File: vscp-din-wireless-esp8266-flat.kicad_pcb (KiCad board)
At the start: 2 copper layers, 64.8 x 51 mm, 25 parts, among them J1 Conn_01x04_Left, J2 Conn_01x04_Right, J3 Conn_01x06, J4 Conn_01x02, Q1 BC547, U2 ESP-12E

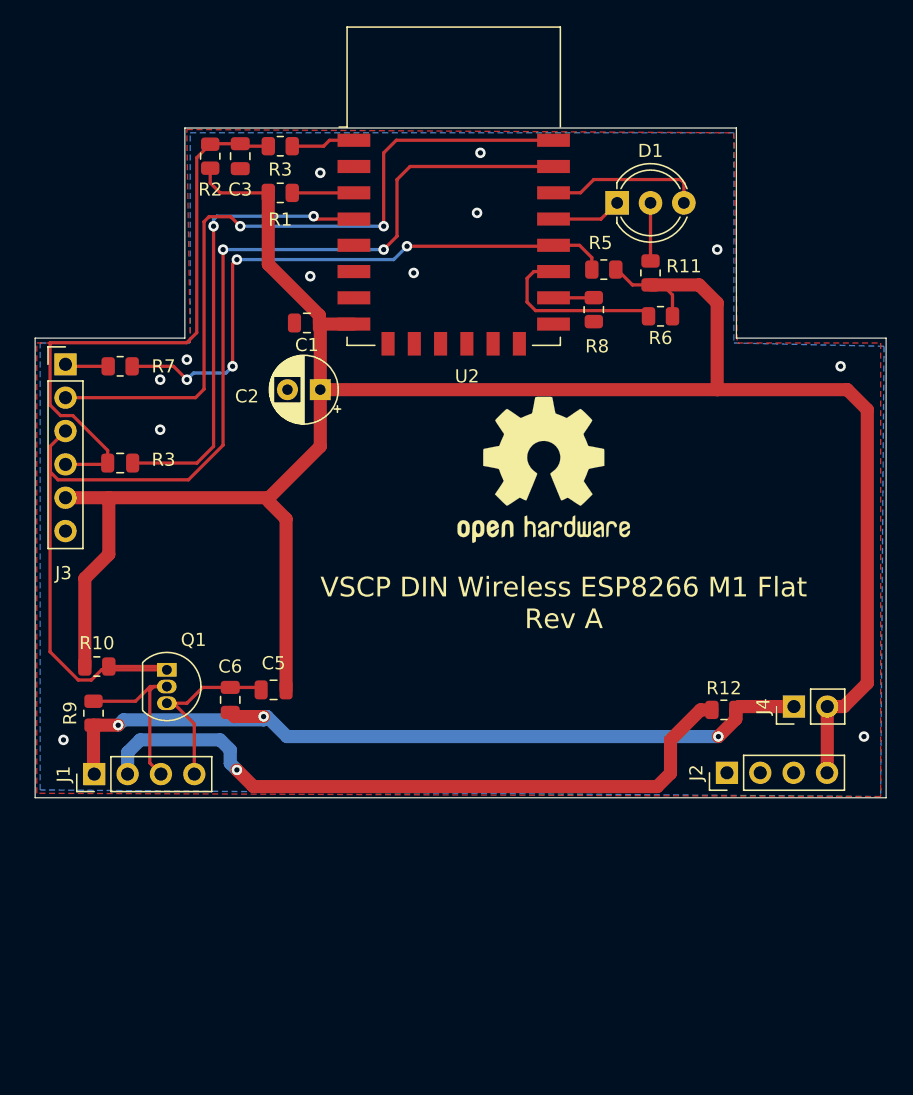
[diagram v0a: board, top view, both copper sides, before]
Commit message: Added gerbers
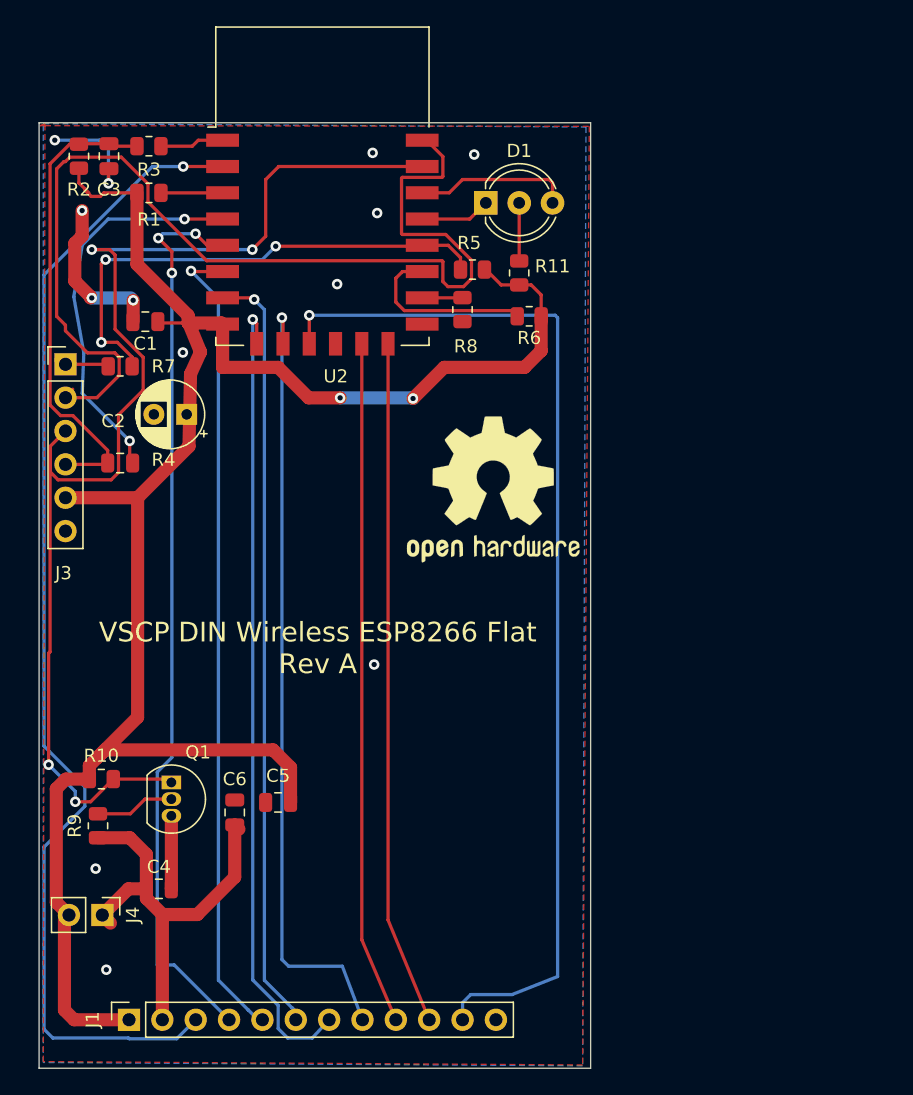
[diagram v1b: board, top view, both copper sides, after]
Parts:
- removed J2: Conn_01x04_Right, Connector_PinHeader_2.54mm:PinHeader_1x04_P2.54mm_Vertical
- removed R12: 0R, Resistor_SMD:R_0805_2012Metric
- added C4: 100nF, Capacitor_SMD:C_0805_2012Metric, F.Cu at (125.1, 106.3)
- J1: value Conn_01x04_Left -> Conn_01x12; footprint Connector_PinHeader_2.54mm:PinHeader_1x04_P2.54mm_Vertical -> Connector_PinSocket_2.54mm:PinSocket_1x12_P2.54mm_Vertical
- moved J4 55.0 mm to (120.8, 108.3), turned to 270 degrees
- moved J1 18.9 mm to (122.8, 116.3)
- moved C1 12.3 mm to (124.1, 63.1)
- moved C2 10.3 mm to (127.2, 70.2)
- moved C3 10.0 mm to (121.3, 50.5)
- moved R1 10.0 mm to (124.4, 53.3)
- moved R2 10.0 mm to (119.0, 50.5)
- moved R3 10.0 mm to (124.4, 49.8)
- moved D1 10.0 mm to (150.0, 54.1)
- moved R11 10.0 mm to (152.6, 59.4)
- moved R5 10.0 mm to (149.0, 59.2)
- moved R6 10.0 mm to (153.3, 62.7)
- moved R8 10.0 mm to (148.2, 62.2)
- moved U2 10.0 mm to (137.6, 52.8)
- moved R10 8.58 mm to (120.7, 98.0)
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- renumbered R3 to R4
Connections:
- J1 pad 1: VDD -> VCC
- J1 pad 2: Net-(J1-Pad2) -> VDD
- J1 pad 3: Net-(J1-Pad3) -> /adc
- J1 pad 4: GND -> /gpio14
- Q1 pad 2: Net-(J1-Pad3) -> /TTLRX
- R9 pad 1: Net-(J1-Pad3) -> /TTLRX
- U2 pad 10: Net-(U2-Pad10) -> /MISO
- U2 pad 11: Net-(U2-Pad11) -> /gpio9
- U2 pad 13: Net-(U2-Pad13) -> /MOSI
- U2 pad 14: Net-(U2-Pad14) -> /SCLK
- U2 pad 2: Net-(U2-Pad2) -> /adc
- U2 pad 5: Net-(U2-Pad5) -> /gpio14
- U2 pad 6: Net-(U2-Pad6) -> /gpio12
- U2 pad 7: Net-(U2-Pad7) -> /gpio13
- U2 pad 9: Net-(U2-Pad9) -> /CS0
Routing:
- net /adc: track 0.00 -> 89.5 mm, vias 0 -> 1
- net /gpio9: track 0.00 -> 80.4 mm, vias 0 -> 1
- net /gpio14: track 0.00 -> 68.8 mm, vias 0 -> 3
- net /gpio12: track 0.00 -> 61.9 mm, vias 0 -> 1
- net /CS0: track 0.00 -> 61.6 mm, vias 0 -> 1
- net /MISO: track 0.00 -> 60.1 mm, vias 0 -> 1
- net /gpio13: track 0.00 -> 58.9 mm, vias 0 -> 1
- net Net-(J1-Pad2): track 52.5 -> 0.00 mm, vias 1 -> 0
- net /SCLK: track 0.00 -> 52.1 mm
- net /MOSI: track 0.00 -> 52.0 mm
- net VDD: track 62.3 -> 33.5 mm, vias 3 -> 0
- net /TXD: track 56.6 -> 81.2 mm, vias 2 -> 0
- net VCC: track 170.2 -> 149.9 mm, vias 0 -> 2
- net Net-(J1-Pad3): track 14.2 -> 0.00 mm
- net GND: track 14.3 -> 26.2 mm, vias 12 -> 13
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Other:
- board size 64.8 x 51 mm -> 42 x 72 mm
- board text added: "VSCP DIN Wireless ESP8266 Flat Rev A"
- board text removed: "VSCP DIN Wireless ESP8266 M1 Flat Rev A"
